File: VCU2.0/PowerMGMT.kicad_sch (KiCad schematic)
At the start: 8 parts, among them IC601 TPS1HA08CQPWPRQ1, IC602 BTS716GB, IC603 BTS716GB, IC604 TPS1HA08CQPWPRQ1

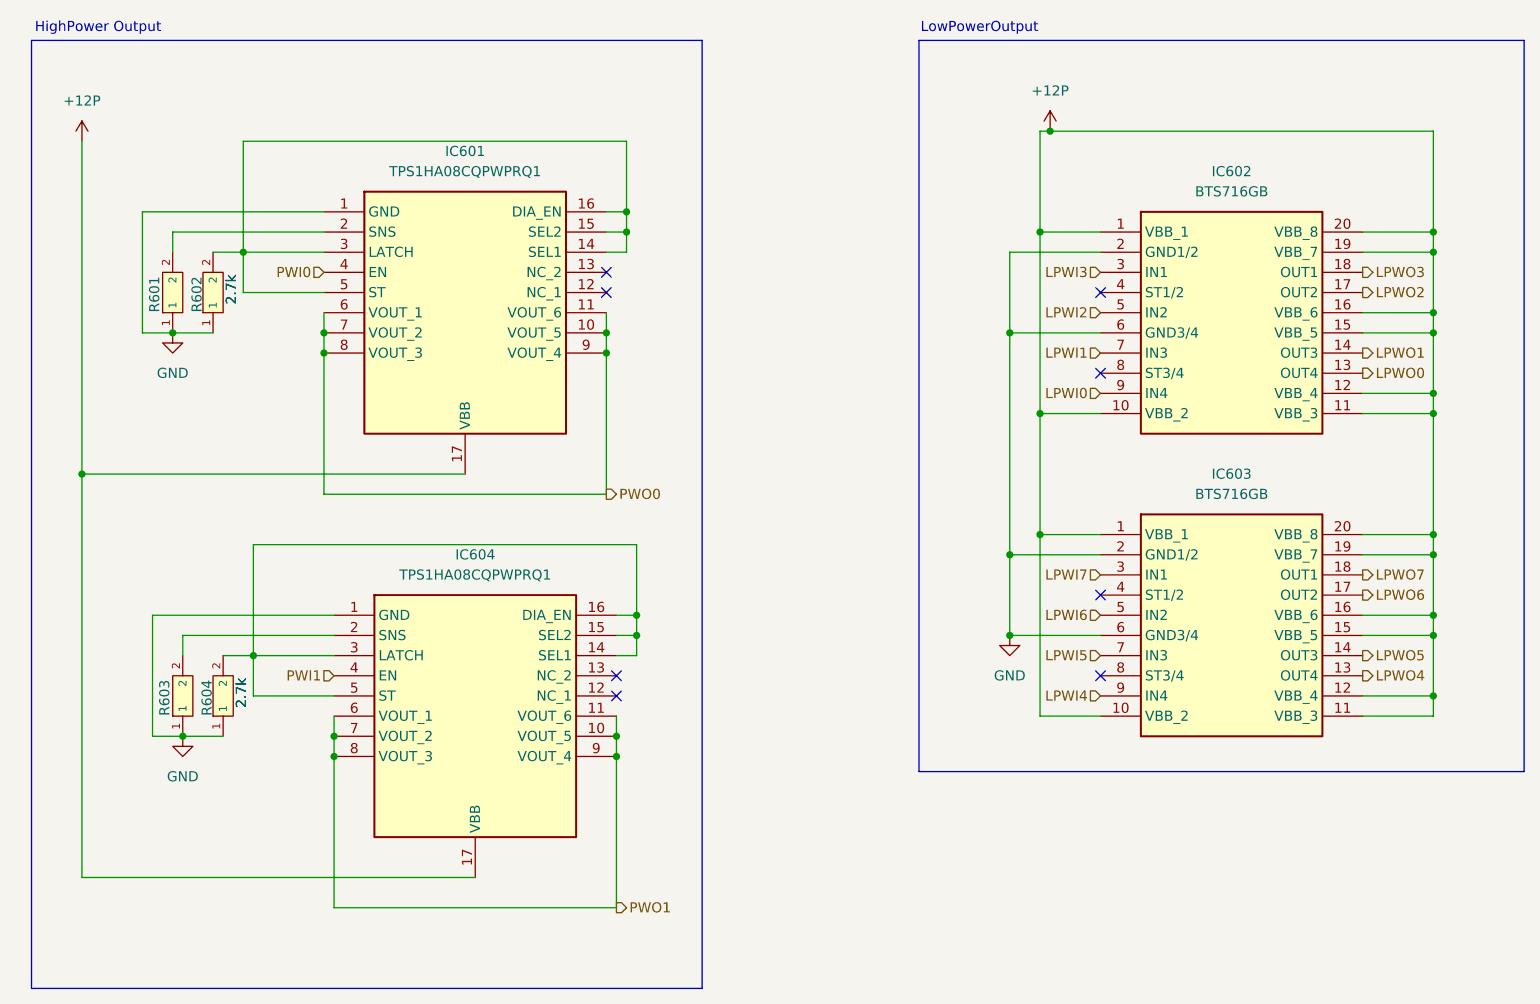
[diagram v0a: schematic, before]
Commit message: current update
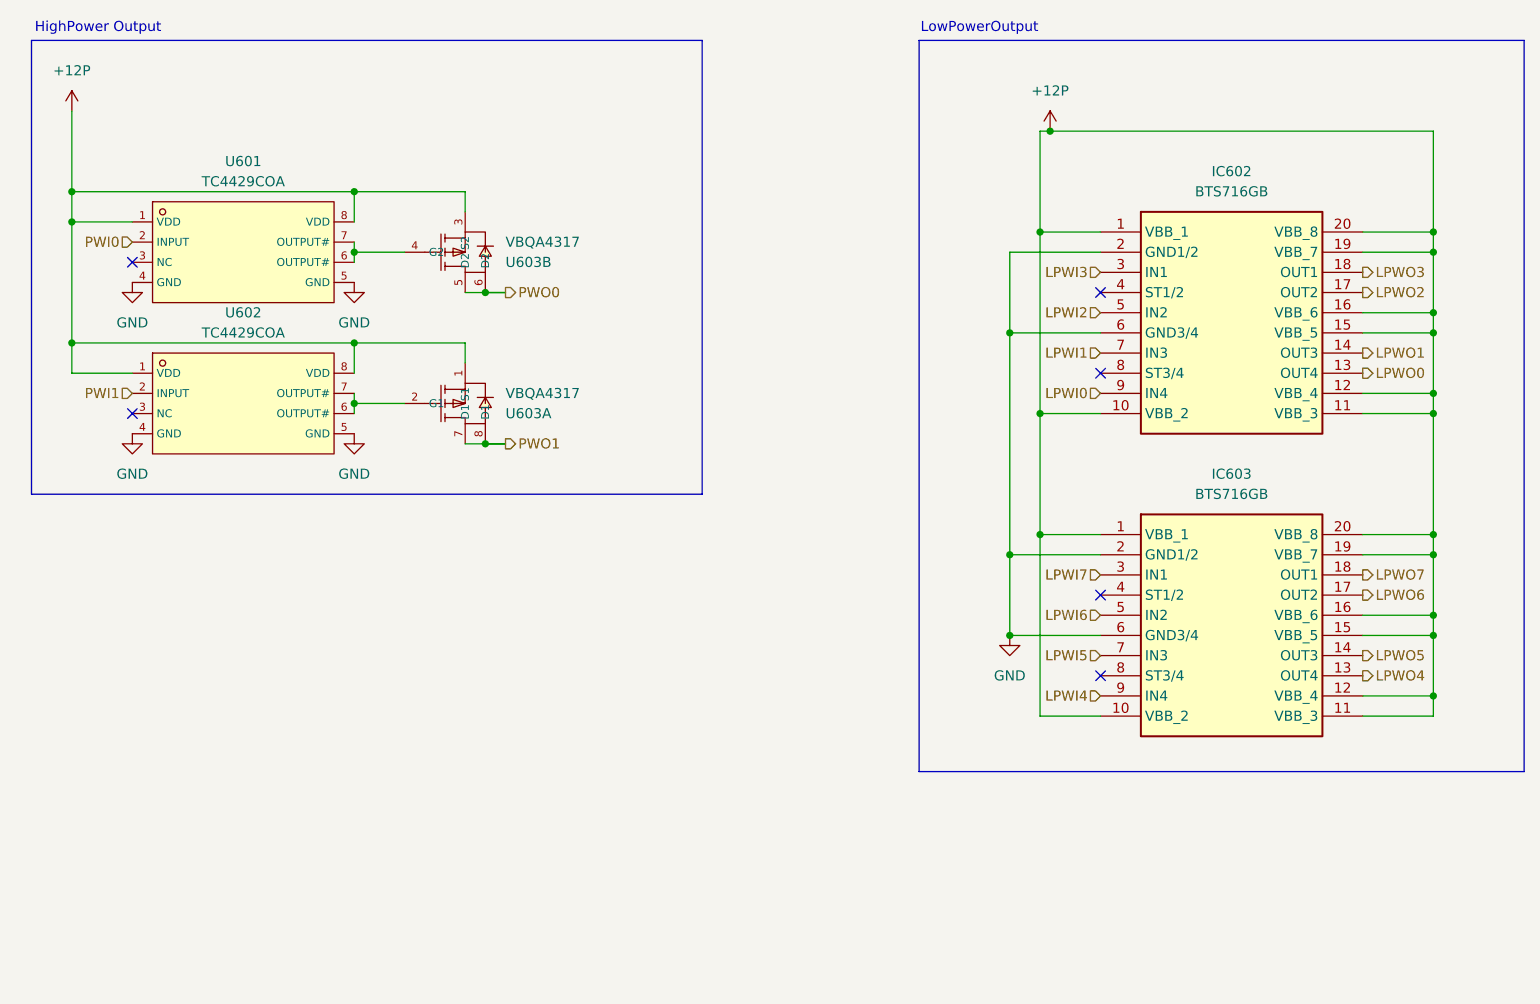
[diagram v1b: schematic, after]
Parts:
- removed IC601, IC604: TPS1HA08CQPWPRQ1, SOP65P640X120-17N, symbol TPS1HA08DQPWPRQ1:TPS1HA08DQPWPRQ1
- removed R601, R602, R603, R604: 2.7k, footprint:R0603, symbol SCR0603J2K7:SCR0603J2K7
- added U601, U602: TC4429COA, footprint:SOIC-8_L4.9-W3.9-P1.27-LS6.0-BL, symbol TC4429COA:TC4429COA
- added U603: VBQA4317, footprint:PDFN-8_L5.9-W5.2-P1.27-LS6.2-BL-1, symbol VBQA4317:VBQA4317
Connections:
- net +12P: now also U601.1 (VDD), U601.8 (VDD), U602.1 (VDD), U602.8 (VDD), U603.1 (S1), U603.3 (S2)
- net GND: now also U601.4 (GND), U601.5 (GND), U602.4 (GND), U602.5 (GND)
- net PWI0: now also U601.2 (INPUT)
- net PWI1: now also U602.2 (INPUT)
- net PWO0: now also U603.5 (D2), U603.6 (D2)
- net PWO1: now also U603.7 (D1), U603.8 (D1)
- new net: U601.6 (OUTPUT#), U601.7 (OUTPUT#), U603.4 (G2)
- new net: U602.6 (OUTPUT#), U602.7 (OUTPUT#), U603.2 (G1)
- no-connect marks 8 -> 6
